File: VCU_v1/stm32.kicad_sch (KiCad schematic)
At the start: 0 parts

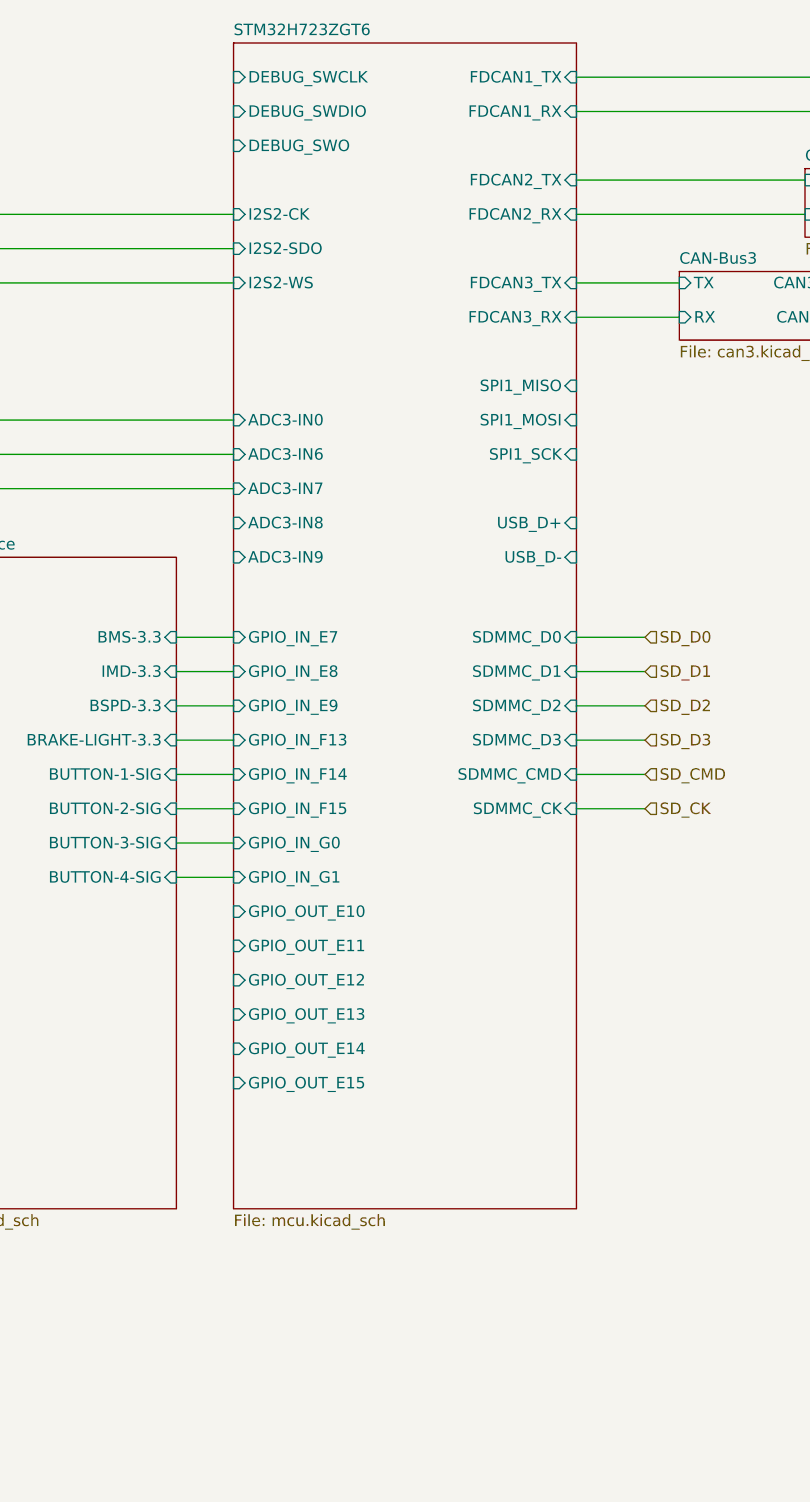
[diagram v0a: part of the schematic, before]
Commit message: left to do before layout: wire DRS/Debug LEDs to connector, add BRUHbus ports
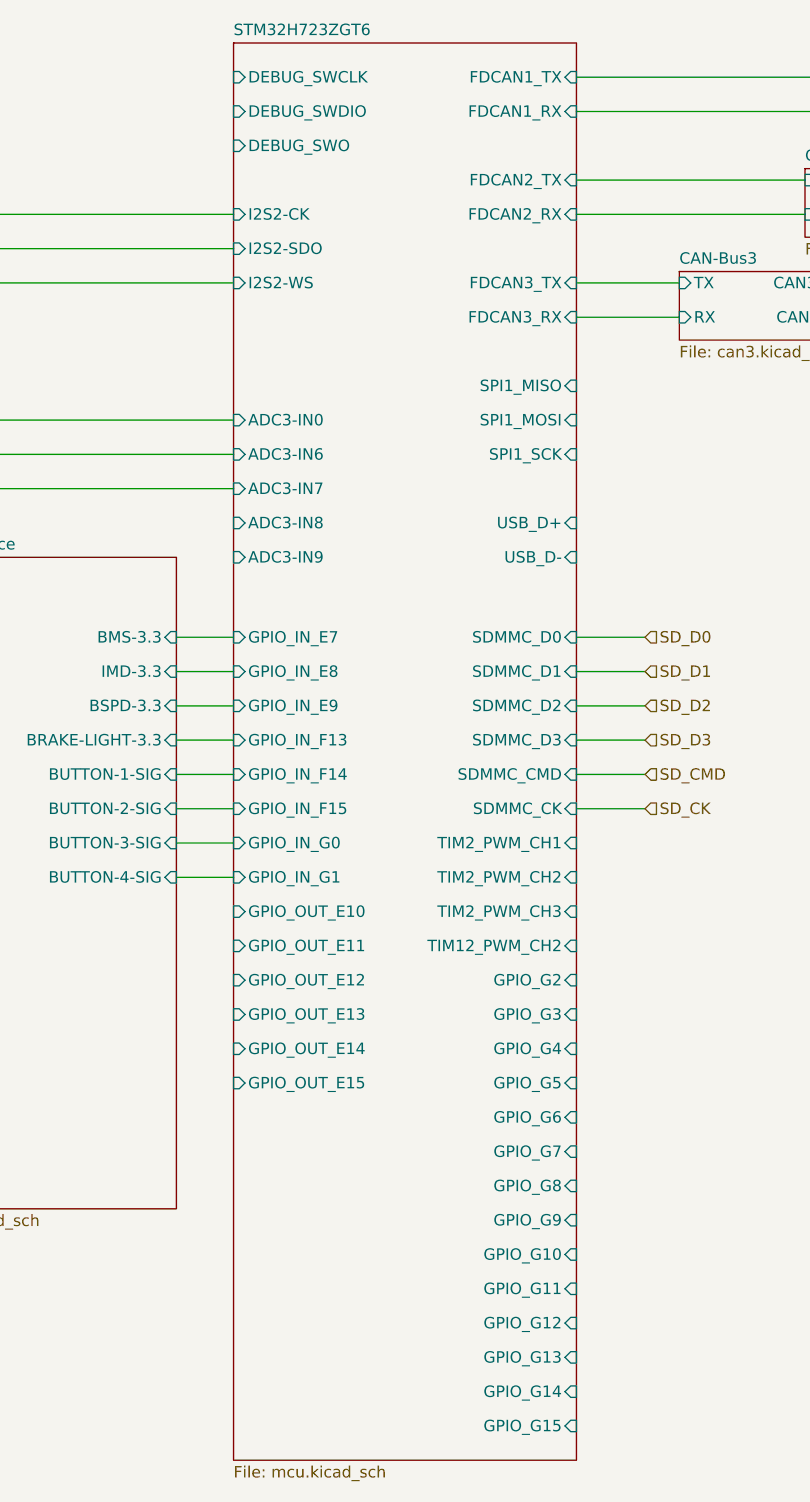
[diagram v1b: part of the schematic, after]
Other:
- sheet STM32H723ZGT6 ports: added GPIO_G10, GPIO_G11, GPIO_G12, GPIO_G13, GPIO_G14, GPIO_G15, GPIO_G2, GPIO_G3, GPIO_G4, GPIO_G5, GPIO_G6, GPIO_G7, GPIO_G8, GPIO_G9, TIM12_PWM_CH2, TIM2_PWM_CH1, TIM2_PWM_CH2, TIM2_PWM_CH3; removed none
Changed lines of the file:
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@@
 	(sheet
 		(at 113.03 40.64)
-		(size 38.1 129.54)
+		(size 38.1 157.48)
 		(exclude_from_sim no)
 		(in_bom yes)
@@
 		)
 		(property "Sheetfile" "mcu.kicad_sch"
-			(at 113.03 170.7646 0)
+			(at 113.03 198.7046 0)
 			(effects
 				(font
@@
 			)
 		)
+		(pin "GPIO_G14" input
+			(at 151.13 190.5 0)
+			(effects
+				(font
+					(size 1.27 1.27)
+				)
+				(justify right)
+			)
+		)
+		(pin "TIM2_PWM_CH1" input
+			(at 151.13 129.54 0)
+			(effects
+				(font
+					(size 1.27 1.27)
+				)
+				(justify right)
+			)
+		)
+		(pin "GPIO_G2" input
+			(at 151.13 144.78 0)
+			(effects
+				(font
+					(size 1.27 1.27)
+				)
+				(justify right)
+			)
+		)
+		(pin "GPIO_G3" input
+			(at 151.13 148.59 0)
+			(effects
+				(font
+					(size 1.27 1.27)
+				)
+				(justify right)
+			)
+		)
+		(pin "GPIO_G5" input
+			(at 151.13 156.21 0)
+			(effects
+				(font
+					(size 1.27 1.27)
+				)
+				(justify right)
+			)
+		)
+		(pin "TIM2_PWM_CH2" input
+			(at 151.13 133.35 0)
+			(effects
+				(font
+					(size 1.27 1.27)
+				)
+				(justify right)
+			)
+		)
+		(pin "GPIO_G4" input
+			(at 151.13 152.4 0)
+			(effects
+				(font
+					(size 1.27 1.27)
+				)
+				(justify right)
+			)
+		)
+		(pin "GPIO_G6" input
+			(at 151.13 160.02 0)
+			(effects
+				(font
+					(size 1.27 1.27)
+				)
+				(justify right)
+			)
+		)
+		(pin "GPIO_G8" input
+			(at 151.13 167.64 0)
+			(effects
+				(font
+					(size 1.27 1.27)
+				)
+				(justify right)
+			)
+		)
+		(pin "GPIO_G7" input
+			(at 151.13 163.83 0)
+			(effects
+				(font
+					(size 1.27 1.27)
+				)
+				(justify right)
+			)
+		)
+		(pin "GPIO_G11" input
+			(at 151.13 179.07 0)
+			(effects
+				(font
+					(size 1.27 1.27)
+				)
+				(justify right)
+			)
+		)
+		(pin "GPIO_G10" input
+			(at 151.13 175.26 0)
+			(effects
+				(font
+					(size 1.27 1.27)
+				)
+				(justify right)
+			)
+		)
+		(pin "GPIO_G9" input
+			(at 151.13 171.45 0)
+			(effects
+				(font
+					(size 1.27 1.27)
+				)
+				(justify right)
+			)
+		)
+		(pin "GPIO_G12" input
+			(at 151.13 182.88 0)
+			(effects
+				(font
+					(size 1.27 1.27)
+				)
+				(justify right)
+			)
+		)
+		(pin "GPIO_G15" input
+			(at 151.13 194.31 0)
+			(effects
+				(font
+					(size 1.27 1.27)
+				)
+				(justify right)
+			)
+		)
+		(pin "GPIO_G13" input
+			(at 151.13 186.69 0)
+			(effects
+				(font
+					(size 1.27 1.27)
+				)
+				(justify right)
+			)
+		)
+		(pin "TIM12_PWM_CH2" input
+			(at 151.13 140.97 0)
+			(effects
+				(font
+					(size 1.27 1.27)
+				)
+				(justify right)
+			)
+		)
+		(pin "TIM2_PWM_CH3" input
+			(at 151.13 137.16 0)
+			(effects
+				(font
+					(size 1.27 1.27)
+				)
+				(justify right)
+			)
+		)
